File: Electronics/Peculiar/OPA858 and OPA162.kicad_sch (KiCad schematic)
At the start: 13 parts, among them U8 ${SIM.PARAMS}, U9 ${SIM.PARAMS}

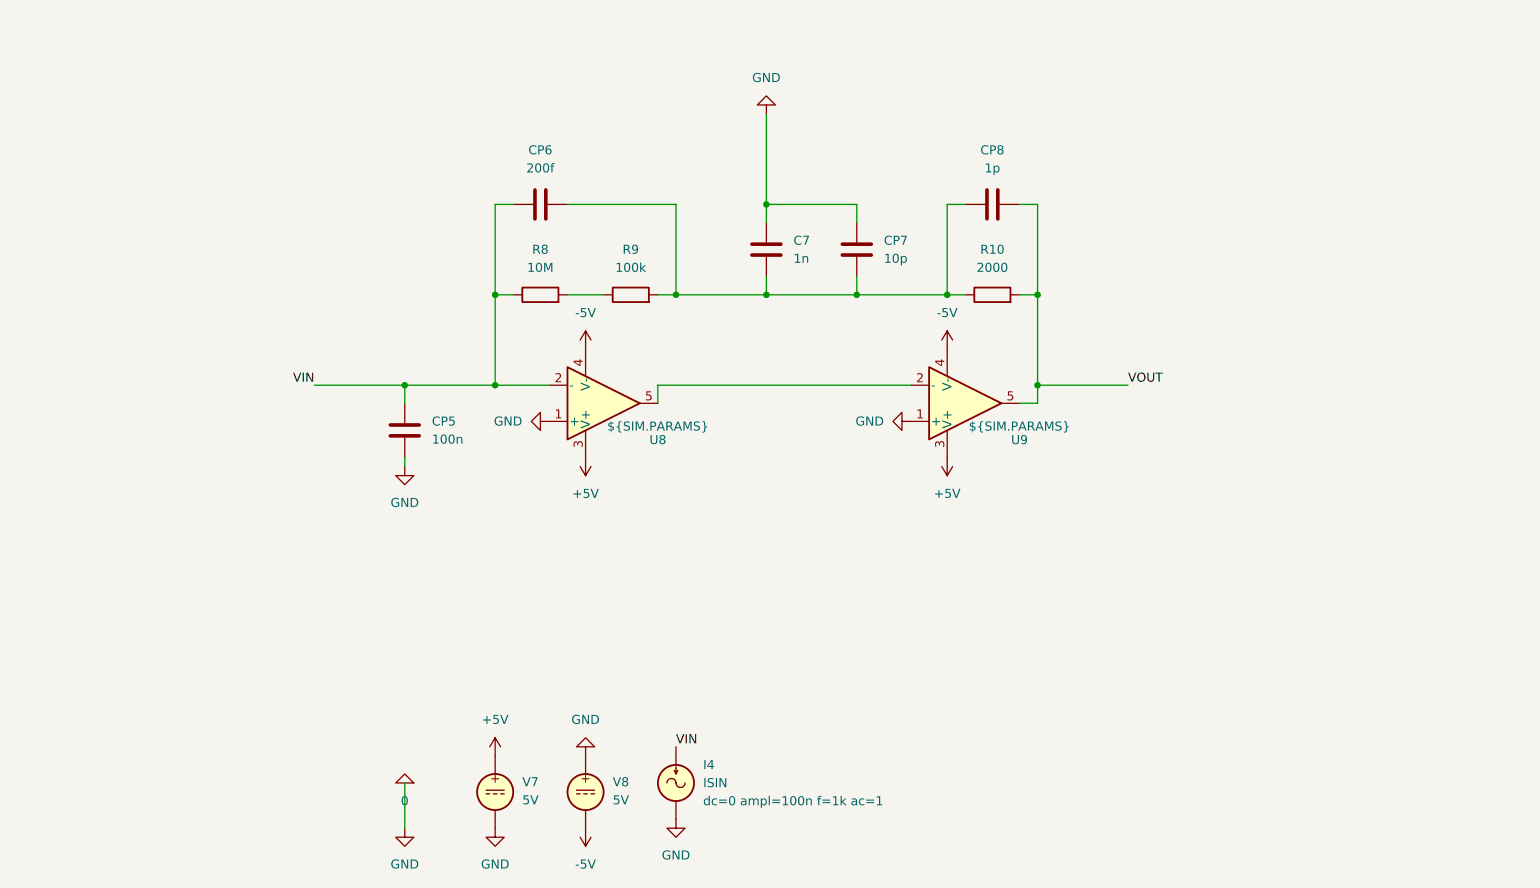
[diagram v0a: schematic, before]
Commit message: Create a great design using OPA858 and OPA162
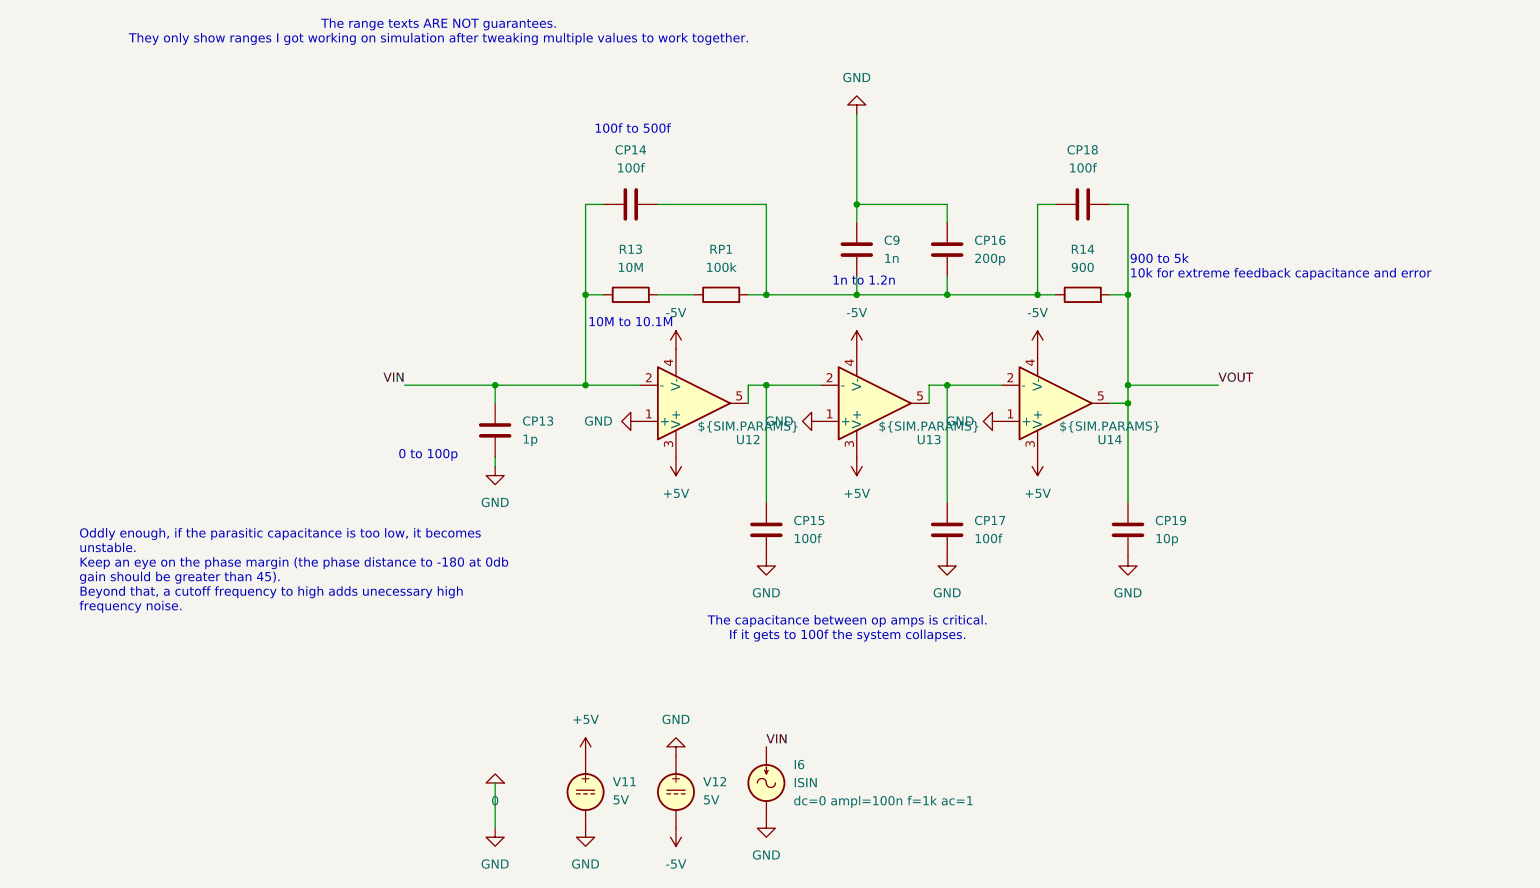
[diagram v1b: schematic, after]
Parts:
- removed C7: 1n, symbol Device:C
- removed CP5: 100n, symbol Device:C
- removed CP6: 200f, symbol Device:C
- removed CP7: 10p, symbol Device:C
- removed CP8: 1p, symbol Device:C
- removed I4: ISIN, symbol Simulation_SPICE:ISIN
- removed R10: 2000, symbol Device:R
- removed R8: 10M, symbol Device:R
- removed R9: 100k, symbol Device:R
- removed U8, U9: ${SIM.PARAMS}, symbol Simulation_SPICE:OPAMP
- removed V7, V8: 5V, symbol Simulation_SPICE:VDC
- added C9: 1n, symbol Device:C
- added CP13: 1p, symbol Device:C
- added CP14, CP15, CP17, CP18: 100f, symbol Device:C
- added CP16: 200p, symbol Device:C
- added CP19: 10p, symbol Device:C
- added I6: ISIN, symbol Simulation_SPICE:ISIN
- added R13: 10M, symbol Device:R
- added R14: 900, symbol Device:R
- added RP1: 100k, symbol Device:R
- added U12, U13, U14: ${SIM.PARAMS}, symbol Simulation_SPICE:OPAMP
- added V11, V12: 5V, symbol Simulation_SPICE:VDC
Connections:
- net +5V: now also U12.3 (V+), U13.3 (V+), U14.3 (V+), V11.1
- net -5V: now also U12.4 (V-), U13.4 (V-), U14.4 (V-), V12.2
- net 0: now also C9.2, CP13.2, CP15.2, CP16.2, CP17.2, CP19.2, I6.2, U12.1 (+), U13.1 (+), U14.1 (+), V11.2, V12.1
- net VIN: now also CP13.1, CP14.1, I6.1, R13.1, U12.2 (-)
- net VOUT: now also CP18.2, CP19.1, R14.2, U14.5
- new net: CP15.1, U12.5, U13.2 (-)
- new net: C9.1, CP14.2, CP16.1, CP18.1, R14.1, RP1.2
- new net: CP17.1, U13.5, U14.2 (-)
- new net: R13.2, RP1.1
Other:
- note added: "0 to 100p"
- note added: "100f to 500f"
- note added: "10M to 10.1M"
- note added: "1n to 1.2n"
- note added: "900 to 5k 10k for extreme feedback capacitance and error"
- note added: "Oddly enough, if the parasitic capacitance is too low, it becomes unstable. Keep an eye on the phase margin (the phase distance to -180 at 0db gain should be greater than 45). Beyond that, a cutoff frequency to high adds unecessary high frequency noise."
- note added: "The capacitance between op amps is critical. If it gets to 100f the system collapses."
- note added: "The range texts ARE NOT guarantees. They only show ranges I got working on simulation after tweaking multiple values to work together."
